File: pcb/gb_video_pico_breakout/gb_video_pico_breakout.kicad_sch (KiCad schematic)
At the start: 19 parts, among them J1 Conn_01x05, U1 SN74LVC1G17QDCKRQ1, U2 SN74LVC1G17QDCKRQ1, U3 SN74LVC1G17QDCKRQ1, U4 Pico

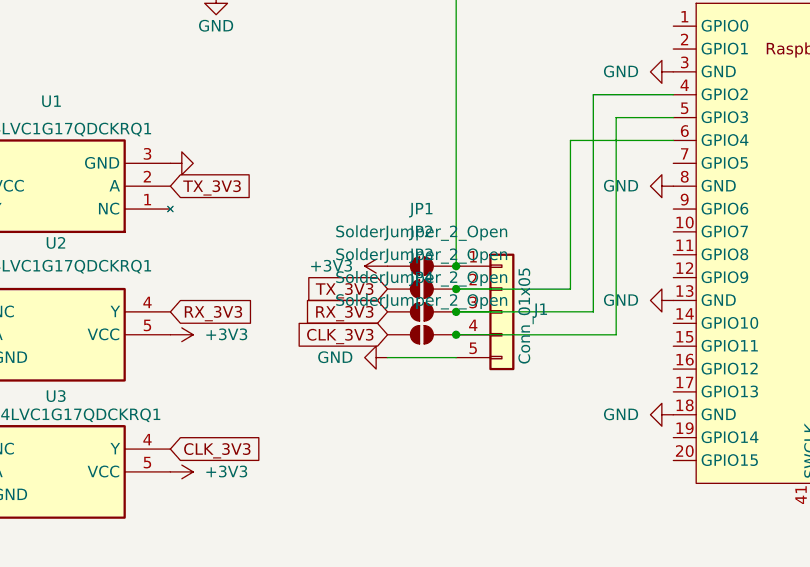
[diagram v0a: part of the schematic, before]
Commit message: add color
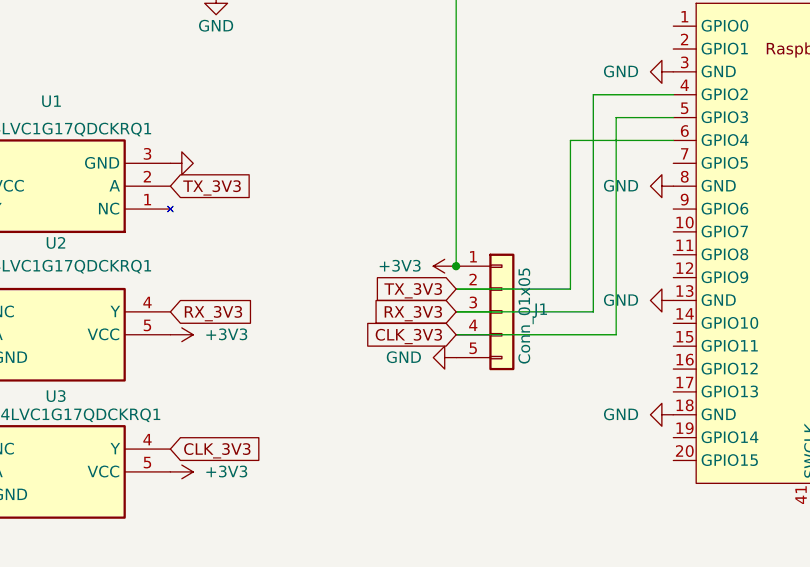
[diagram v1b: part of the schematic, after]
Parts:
- removed JP1, JP2, JP3, JP4: SolderJumper_2_Open, Jumper:SolderJumper-2_P1.3mm_Open_RoundedPad1.0x1.5mm, symbol Jumper:SolderJumper_2_Open
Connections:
- net +3V3: now also J1.1 (Pin_1), U4.36 (3V3)
- net CLK_3V3: now also J1.4 (Pin_4), U4.5 (GPIO3)
- net RX_3V3: now also J1.3 (Pin_3), U4.4 (GPIO2)
- net TX_3V3: now also J1.2 (Pin_2), U4.6 (GPIO4)
